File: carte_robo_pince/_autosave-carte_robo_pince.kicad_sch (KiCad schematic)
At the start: 17 parts, among them J1 Conn_01x18_Pin, J2 Conn_01x18_Pin, J3 Conn_01x03_Socket, J4 Conn_01x03_Socket, J5 Conn_01x03_Socket, J6 Conn_01x03_Socket, J7 Conn_01x03_Socket, SW1 SW_DIP_x01, U1 KA78M05_TO252

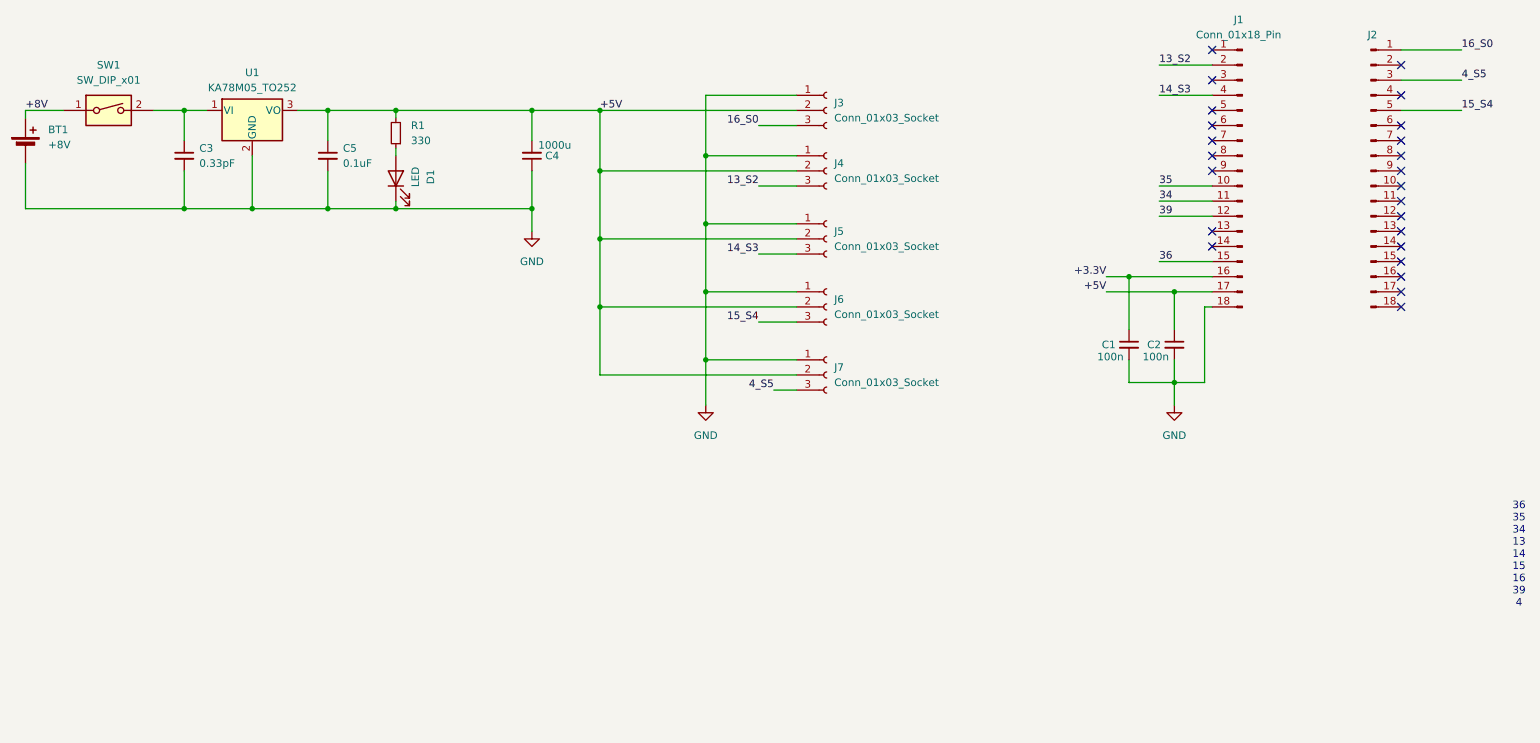
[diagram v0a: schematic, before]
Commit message: 19/03
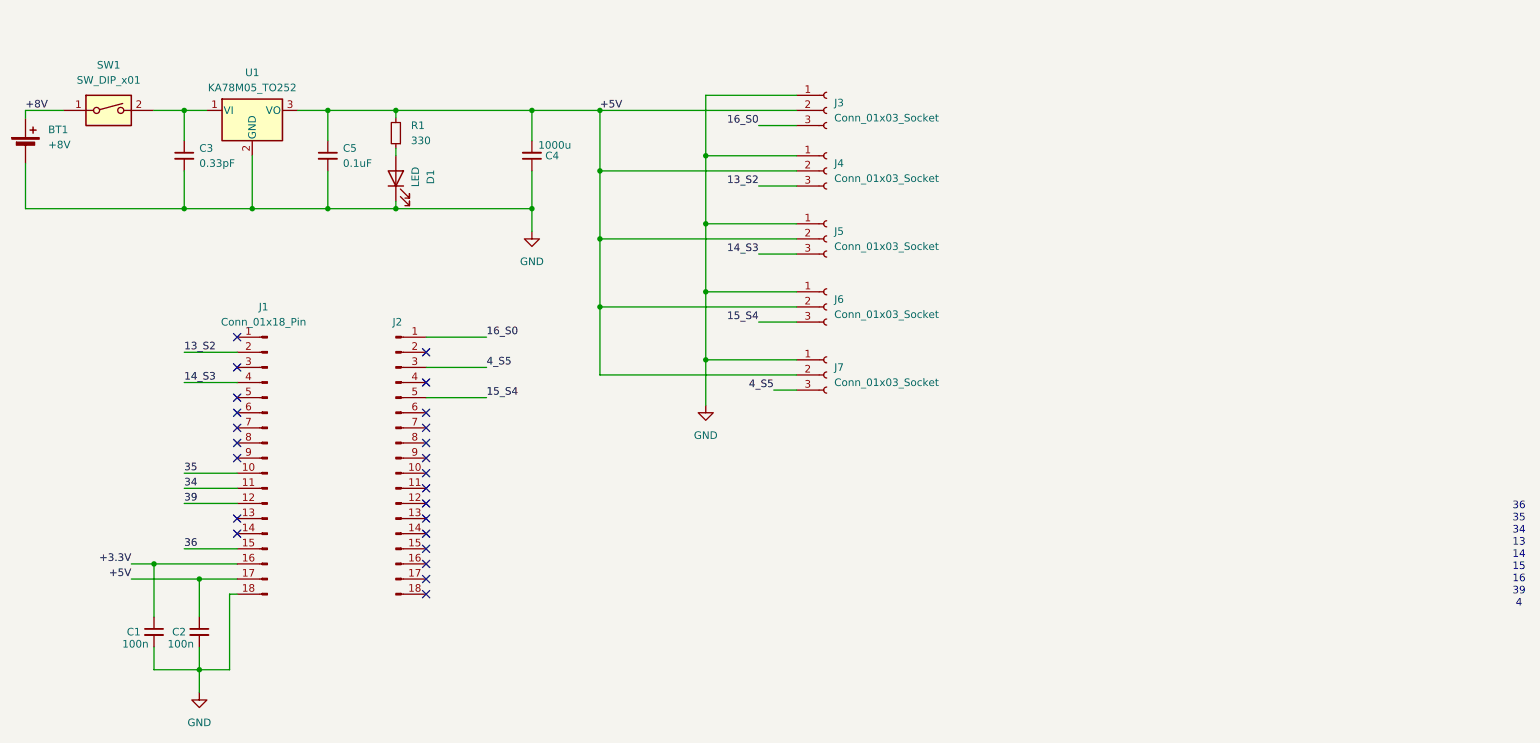
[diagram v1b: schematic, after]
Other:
- moved on the sheet: C1, C2, J1, J2
